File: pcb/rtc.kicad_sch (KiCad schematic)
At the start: 4 parts, among them U1 bq3285, U2 Socket, Y1 32.768kHz 6pF

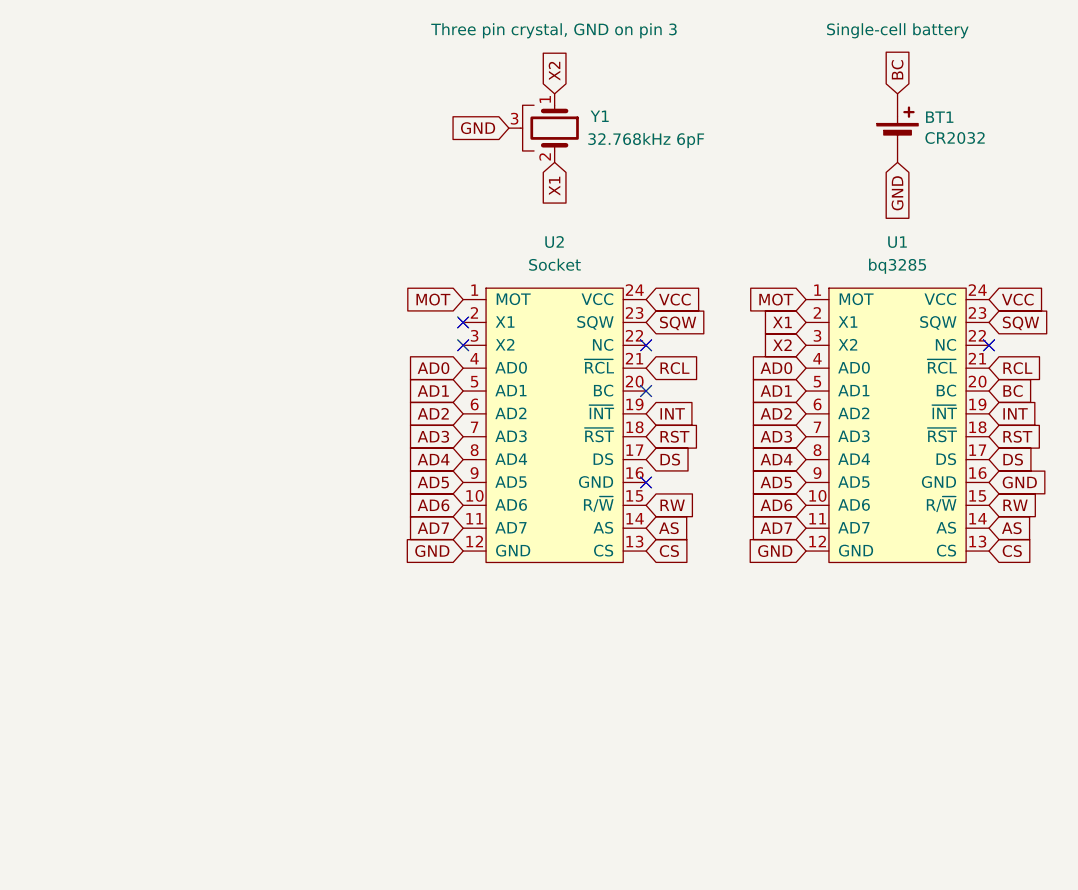
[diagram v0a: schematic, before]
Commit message: rename project, remove unused files, change info
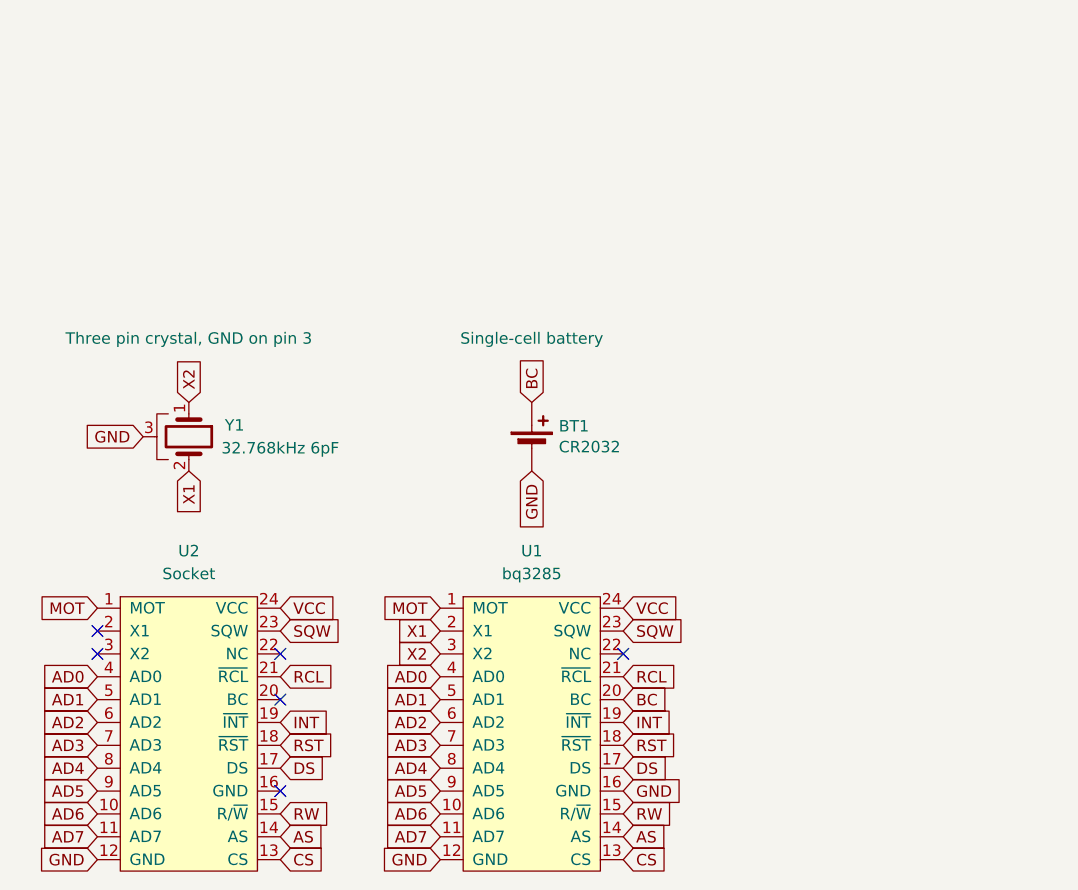
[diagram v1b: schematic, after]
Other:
- company: Necroware -> CityRunner
- title: nwX287.2032.ssop -> rtc-cr2032-ssop
- moved on the sheet: BT1, U1, U2, Y1

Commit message: adjustments
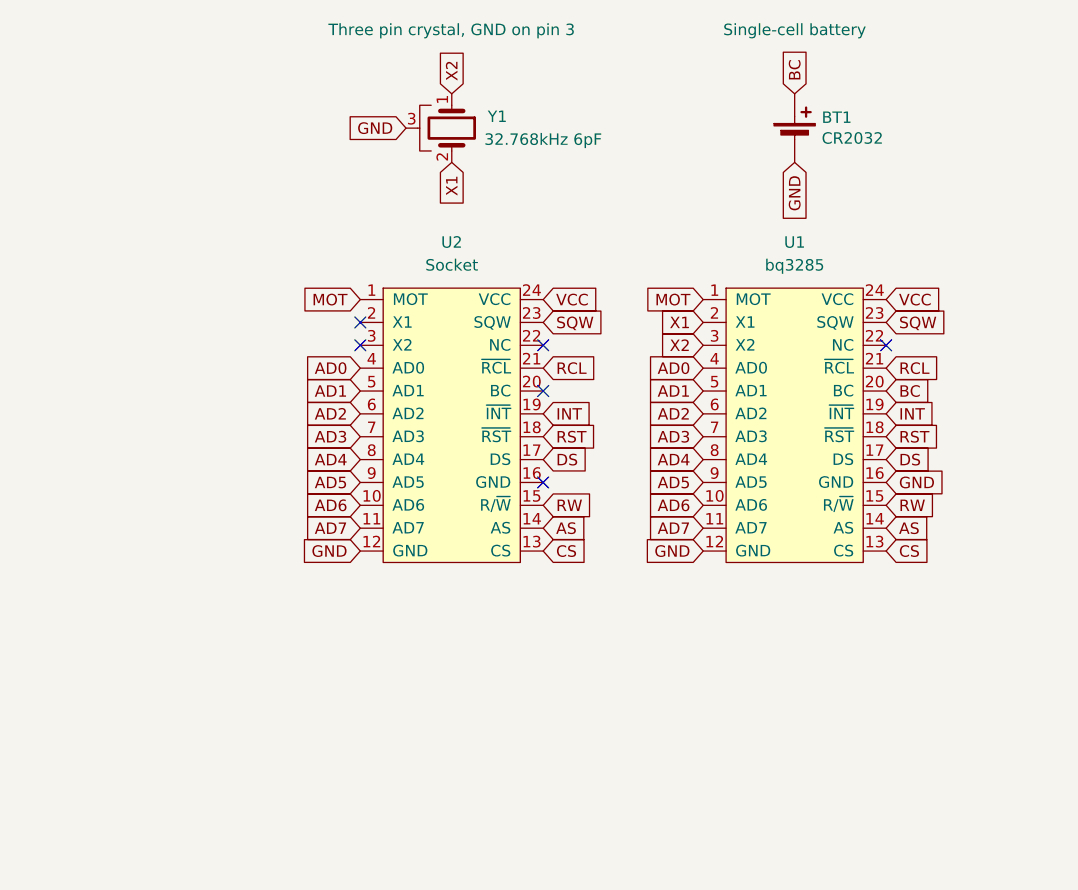
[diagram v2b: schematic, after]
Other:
- title: rtc-cr2032-ssop -> rtc-int-cr2032
- moved on the sheet: BT1, U1, U2, Y1
